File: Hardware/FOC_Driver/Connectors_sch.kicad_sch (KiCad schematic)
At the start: 15 parts, among them J1 USB_C_Receptacle_USB2.0_16P, J2 MR30, J4 XT30, J5 Conn_ARM_SWD_TagConnect_TC203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, J6 TestPoint, J7 TestPoint, J8 TestPoint, U2 USBLC6-2SC6

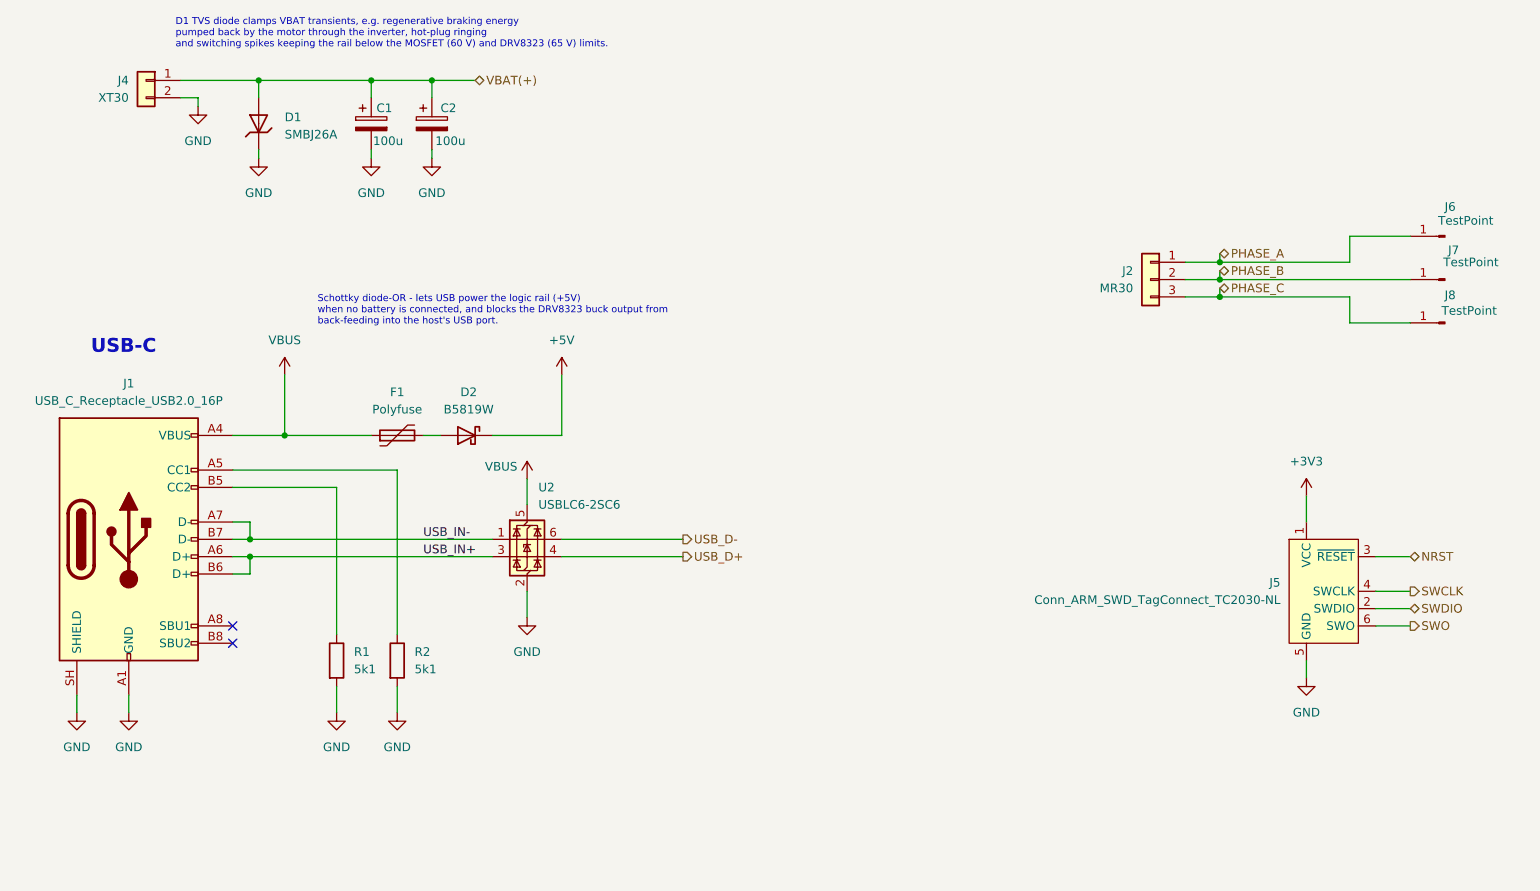
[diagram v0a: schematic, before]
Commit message: schematic updates
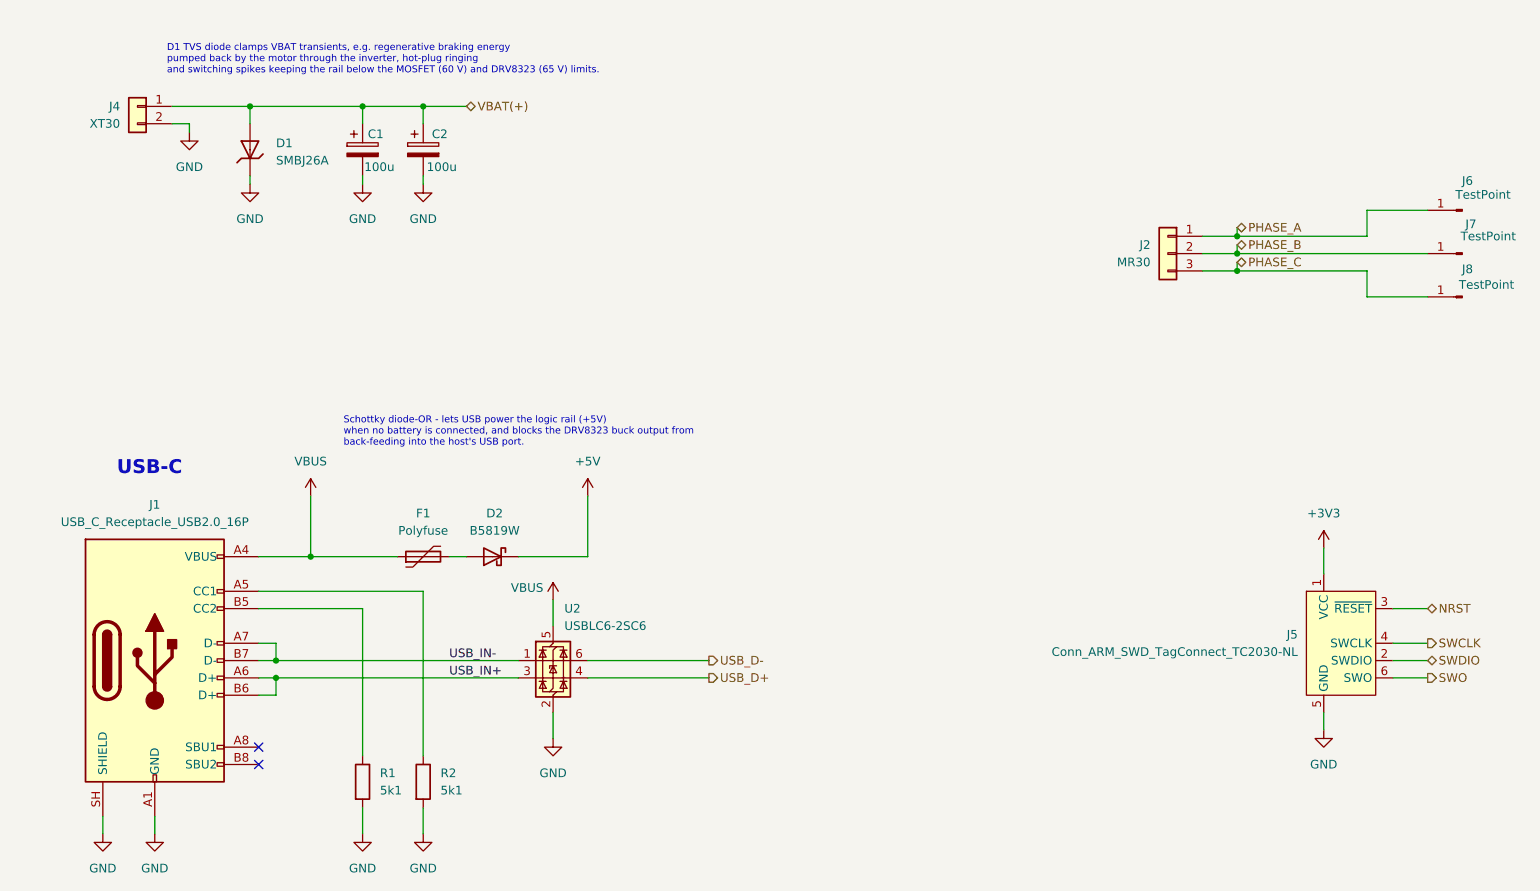
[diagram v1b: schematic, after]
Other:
- moved on the sheet: C1, C2, D1, D2, F1, J1, J2, J4, J5, J6, J7, J8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
